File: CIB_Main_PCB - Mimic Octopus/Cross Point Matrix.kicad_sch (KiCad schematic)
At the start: 6 parts, among them J10 Ch 5-8, J11 Ch 9-12, J12 Ch 13-16, J13 Ch 17-20, J14 Ch 21-24, J9 Ch 1-4

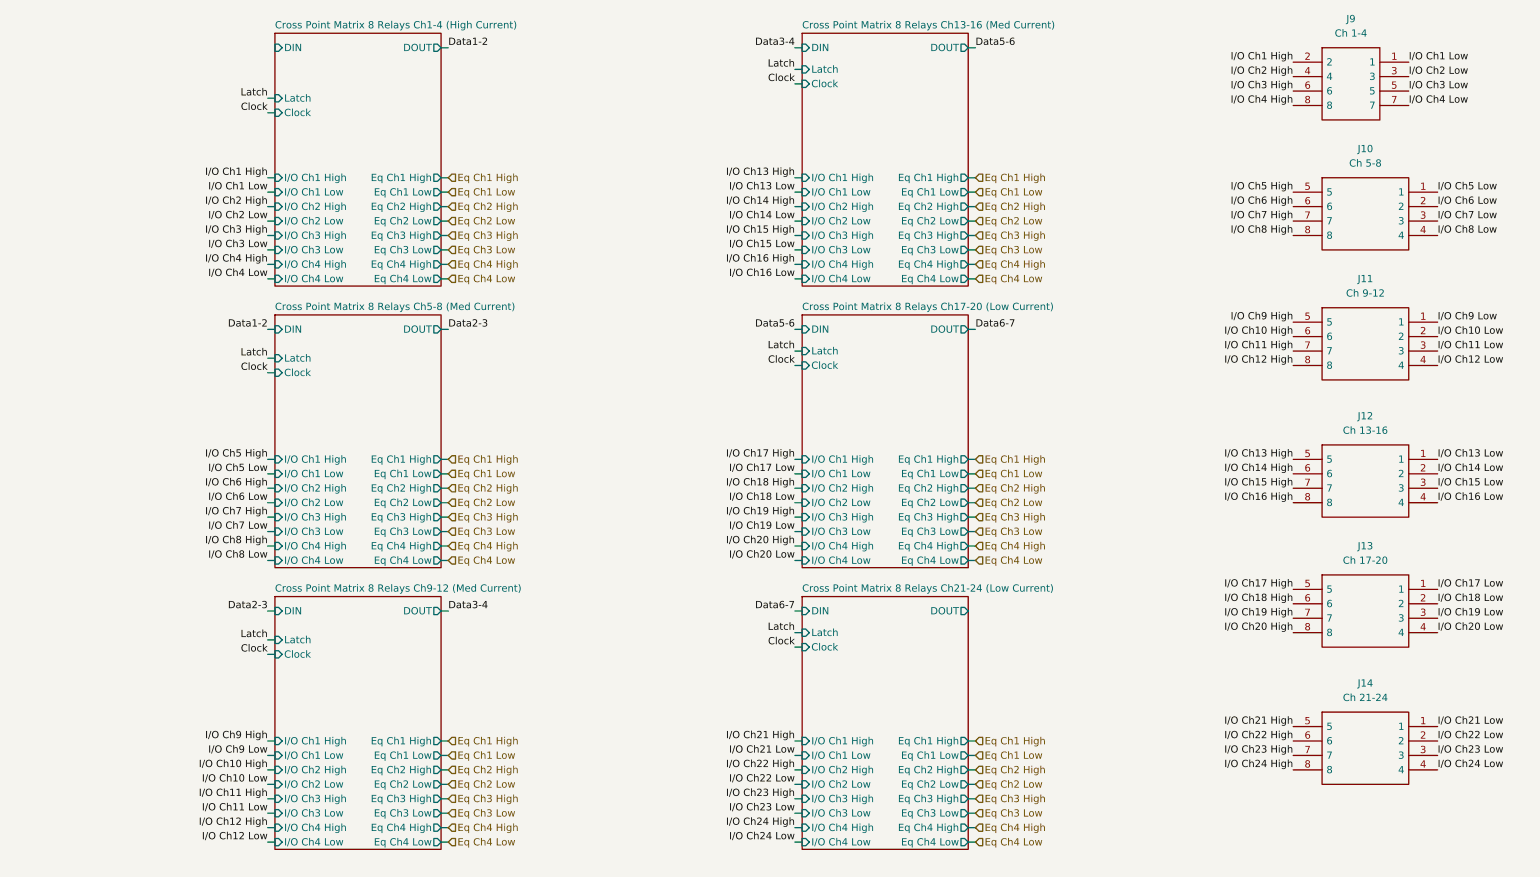
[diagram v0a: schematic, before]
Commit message: V0.1 PCB to be sent out
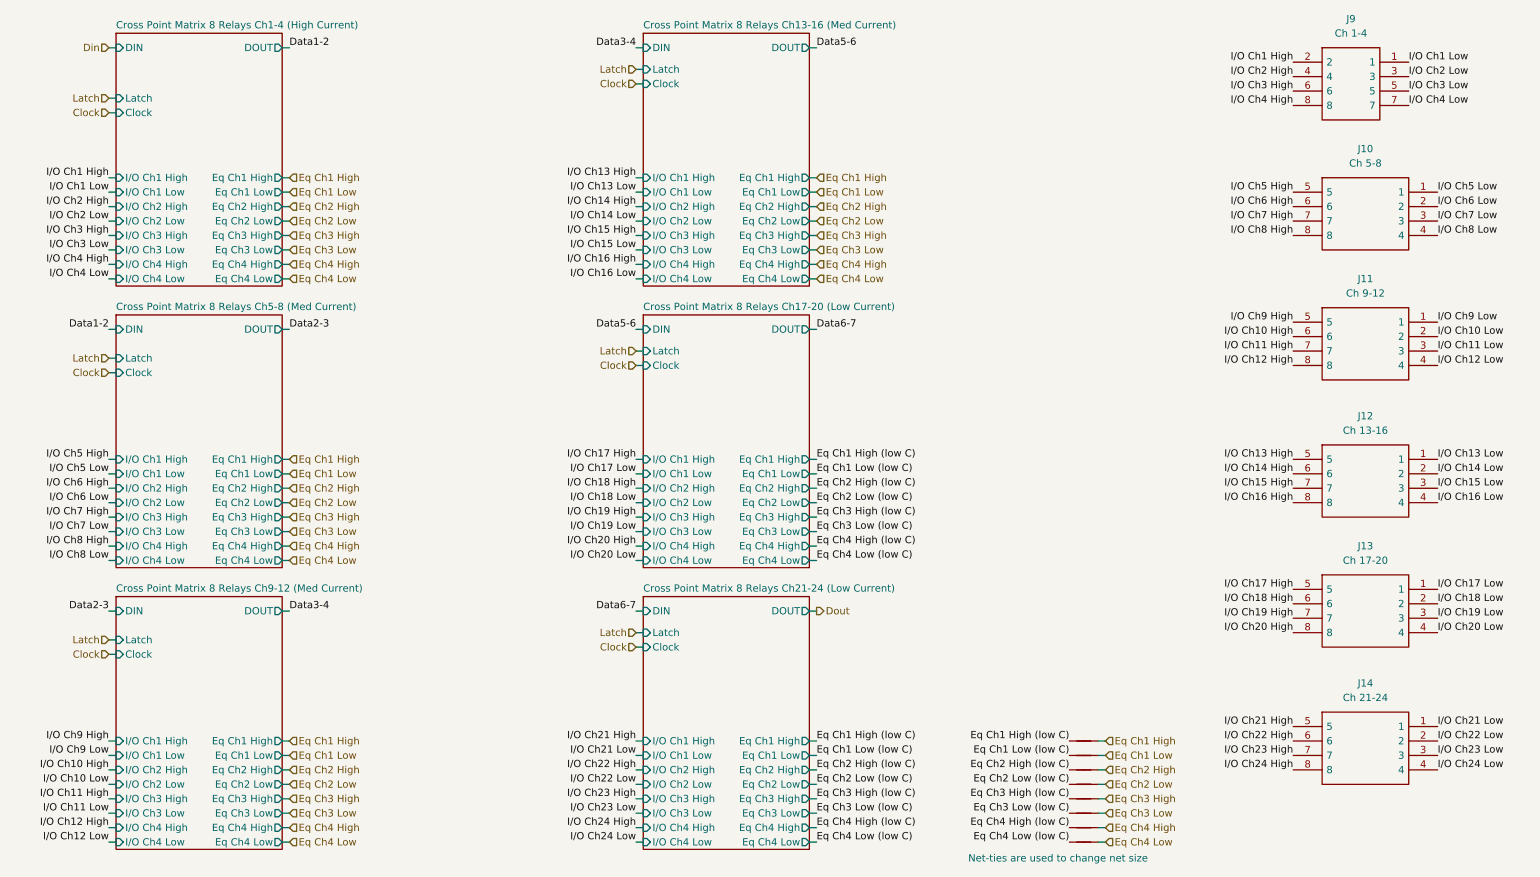
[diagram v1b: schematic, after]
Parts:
- added NT1, NT2, NT3, NT4, NT5, NT6, NT7, NT8: NetTie_2, NetTie:NetTie-2_SMD_Pad0.5mm, symbol Device:NetTie_2
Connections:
- net Eq Ch1 High: now also NT1.2
- net Eq Ch1 Low: now also NT2.2
- net Eq Ch2 High: now also NT3.2
- net Eq Ch2 Low: now also NT4.2
- net Eq Ch3 High: now also NT5.2
- net Eq Ch3 Low: now also NT6.2
- net Eq Ch4 High: now also NT7.2
- net Eq Ch4 Low: now also NT8.2
- new net Eq Ch1 High (low C): NT1.1
- new net Eq Ch1 Low (low C): NT2.1
- new net Eq Ch2 High (low C): NT3.1
- new net Eq Ch2 Low (low C): NT4.1
- new net Eq Ch3 High (low C): NT5.1
- new net Eq Ch3 Low (low C): NT6.1
- new net Eq Ch4 High (low C): NT7.1
- new net Eq Ch4 Low (low C): NT8.1
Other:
- note added: "Net-ties are used to change net size"

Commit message: BoM
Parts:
- J10, J11, J12, J13, J14: Manufacturer_Name Phoenix Contact -> (none); Manufacturer_Part_Number 1848668 -> (none); Mouser # (none) -> 651-1848668; Mouser Part Number 651-1848668 -> (none)
- J9: Manufacturer_Name Phoenix Contact -> (none); Manufacturer_Part_Number 1864095 -> (none); Mouser # (none) -> 651-1864095; Mouser Part Number 651-1864095 -> (none)
- NT1, NT2, NT3, NT4, NT5, NT6, NT7, NT8: dnp (none) -> dnp
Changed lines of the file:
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@@
+      (effects (font (size 1.27 1.27)) hide)
+    )
+    (property "dnp" "dnp" (id 4) (at 204.47 156.21 0)
       (effects (font (size 1.27 1.27)) hide)
     )
@@
       (effects (font (size 1.27 1.27)) (justify left) hide)
     )
-    (property "Manufacturer_Name" "Phoenix Contact" (id 6) (at 262.89 101.6 0)
-      (effects (font (size 1.27 1.27)) (justify left) hide)
-    )
-    (property "Manufacturer_Part_Number" "1848668" (id 7) (at 262.89 104.14 0)
-      (effects (font (size 1.27 1.27)) (justify left) hide)
-    )
-    (property "Mouser Part Number" "651-1848668" (id 8) (at 262.89 106.68 0)
+    (property "Manufacturer_Name" "" (id 6) (at 262.89 101.6 0)
+      (effects (font (size 1.27 1.27)) (justify left) hide)
+    )
+    (property "Manufacturer_Part_Number" "" (id 7) (at 262.89 104.14 0)
+      (effects (font (size 1.27 1.27)) (justify left) hide)
+    )
+    (property "Mouser Part Number" "" (id 8) (at 262.89 106.68 0)
       (effects (font (size 1.27 1.27)) (justify left) hide)
     )
@@
     )
     (property "Manufacturer #" "1848668" (id 13) (at 241.3 93.98 0)
+      (effects (font (size 1.27 1.27)) hide)
+    )
+    (property "Mouser #" "651-1848668" (id 14) (at 241.3 93.98 0)
       (effects (font (size 1.27 1.27)) hide)
     )
@@
       (effects (font (size 1.27 1.27)) (justify left) hide)
     )
-    (property "Manufacturer_Name" "Phoenix Contact" (id 6) (at 262.89 54.61 0)
-      (effects (font (size 1.27 1.27)) (justify left) hide)
-    )
-    (property "Manufacturer_Part_Number" "1848668" (id 7) (at 262.89 57.15 0)
-      (effects (font (size 1.27 1.27)) (justify left) hide)
-    )
-    (property "Mouser Part Number" "651-1848668" (id 8) (at 262.89 59.69 0)
+    (property "Manufacturer_Name" "" (id 6) (at 262.89 54.61 0)
+      (effects (font (size 1.27 1.27)) (justify left) hide)
+    )
+    (property "Manufacturer_Part_Number" "" (id 7) (at 262.89 57.15 0)
+      (effects (font (size 1.27 1.27)) (justify left) hide)
+    )
+    (property "Mouser Part Number" "" (id 8) (at 262.89 59.69 0)
       (effects (font (size 1.27 1.27)) (justify left) hide)
     )
@@
     )
     (property "Manufacturer #" "1848668" (id 13) (at 241.3 46.99 0)
+      (effects (font (size 1.27 1.27)) hide)
+    )
+    (property "Mouser #" "651-1848668" (id 14) (at 241.3 46.99 0)
       (effects (font (size 1.27 1.27)) hide)
     )
@@
       (effects (font (size 1.27 1.27)) hide)
     )
+    (property "dnp" "dnp" (id 4) (at 204.47 158.75 0)
+      (effects (font (size 1.27 1.27)) hide)
+    )
     (pin "1")
     (pin "2")
@@
       (effects (font (size 1.27 1.27)) hide)
     )
+    (property "dnp" "dnp" (id 4) (at 204.47 143.51 0)
+      (effects (font (size 1.27 1.27)) hide)
+    )
     (pin "1")
     (pin "2")
@@
       (effects (font (size 1.27 1.27)) hide)
     )
+    (property "dnp" "dnp" (id 4) (at 204.47 151.13 0)
+      (effects (font (size 1.27 1.27)) hide)
+    )
     (pin "1")
     (pin "2")
@@
       (effects (font (size 1.27 1.27)) hide)
     )
+    (property "dnp" "dnp" (id 4) (at 204.47 161.29 0)
+      (effects (font (size 1.27 1.27)) hide)
+    )
     (pin "1")
     (pin "2")
@@
     )
     (property "Datasheet" "~" (id 3) (at 204.47 153.67 0)
+      (effects (font (size 1.27 1.27)) hide)
+    )
+    (property "dnp" "dnp" (id 4) (at 204.47 153.67 0)
       (effects (font (size 1.27 1.27)) hide)
     )
@@
       (effects (font (size 1.27 1.27)) (justify left) hide)
     )
-    (property "Manufacturer_Name" "Phoenix Contact" (id 6) (at 262.89 124.46 0)
-      (effects (font (size 1.27 1.27)) (justify left) hide)
-    )
-    (property "Manufacturer_Part_Number" "1848668" (id 7) (at 262.89 127 0)
-      (effects (font (size 1.27 1.27)) (justify left) hide)
-    )
-    (property "Mouser Part Number" "651-1848668" (id 8) (at 262.89 129.54 0)
+    (property "Manufacturer_Name" "" (id 6) (at 262.89 124.46 0)
+      (effects (font (size 1.27 1.27)) (justify left) hide)
+    )
+    (property "Manufacturer_Part_Number" "" (id 7) (at 262.89 127 0)
+      (effects (font (size 1.27 1.27)) (justify left) hide)
+    )
+    (property "Mouser Part Number" "" (id 8) (at 262.89 129.54 0)
       (effects (font (size 1.27 1.27)) (justify left) hide)
     )
@@
     )
     (property "Manufacturer #" "1848668" (id 13) (at 241.3 116.84 0)
+      (effects (font (size 1.27 1.27)) hide)
+    )
+    (property "Mouser #" "651-1848668" (id 14) (at 241.3 116.84 0)
       (effects (font (size 1.27 1.27)) hide)
     )
@@
       (effects (font (size 1.27 1.27)) (justify left) hide)
     )
-    (property "Description" "Push spring connector 5mm pitch 8 way Phoenix Contact SDC Series 5mm Pitch Straight Pluggable Terminal Block, Plug with Plug In Termination, PCB Mount, 8 Way" (id 4) (at 257.81 26.67 0)
+    (property "Description" "Pluggable Terminal Blocks SDDC 1,5/ 4-PV-3,5" (id 4) (at 257.81 26.67 0)
       (effects (font (size 1.27 1.27)) (justify left) hide)
     )
@@
       (effects (font (size 1.27 1.27)) (justify left) hide)
     )
-    (property "Manufacturer_Name" "Phoenix Contact" (id 6) (at 257.81 31.75 0)
-      (effects (font (size 1.27 1.27)) (justify left) hide)
-    )
-    (property "Manufacturer_Part_Number" "1864095" (id 7) (at 257.81 34.29 0)
-      (effects (font (size 1.27 1.27)) (justify left) hide)
-    )
-    (property "Mouser Part Number" "651-1864095" (id 8) (at 257.81 36.83 0)
+    (property "Manufacturer_Name" "" (id 6) (at 257.81 31.75 0)
+      (effects (font (size 1.27 1.27)) (justify left) hide)
+    )
+    (property "Manufacturer_Part_Number" "" (id 7) (at 257.81 34.29 0)
+      (effects (font (size 1.27 1.27)) (justify left) hide)
+    )
+    (property "Mouser Part Number" "" (id 8) (at 257.81 36.83 0)
       (effects (font (size 1.27 1.27)) (justify left) hide)
     )
@@
     )
     (property "Manufacturer #" "1864095" (id 13) (at 241.3 24.13 0)
+      (effects (font (size 1.27 1.27)) hide)
+    )
+    (property "Mouser #" "651-1864095" (id 14) (at 241.3 24.13 0)
       (effects (font (size 1.27 1.27)) hide)
     )
@@
       (effects (font (size 1.27 1.27)) hide)
     )
+    (property "dnp" "dnp" (id 4) (at 204.47 146.05 0)
+      (effects (font (size 1.27 1.27)) hide)
+    )
     (pin "1")
     (pin "2")
@@
       (effects (font (size 1.27 1.27)) (justify left) hide)
     )
-    (property "Manufacturer_Name" "Phoenix Contact" (id 6) (at 262.89 148.59 0)
-      (effects (font (size 1.27 1.27)) (justify left) hide)
-    )
-    (property "Manufacturer_Part_Number" "1848668" (id 7) (at 262.89 151.13 0)
-      (effects (font (size 1.27 1.27)) (justify left) hide)
-    )
-    (property "Mouser Part Number" "651-1848668" (id 8) (at 262.89 153.67 0)
+    (property "Manufacturer_Name" "" (id 6) (at 262.89 148.59 0)
+      (effects (font (size 1.27 1.27)) (justify left) hide)
+    )
+    (property "Manufacturer_Part_Number" "" (id 7) (at 262.89 151.13 0)
+      (effects (font (size 1.27 1.27)) (justify left) hide)
+    )
+    (property "Mouser Part Number" "" (id 8) (at 262.89 153.67 0)
       (effects (font (size 1.27 1.27)) (justify left) hide)
     )
@@
     )
     (property "Manufacturer #" "1848668" (id 13) (at 241.3 140.97 0)
+      (effects (font (size 1.27 1.27)) hide)
+    )
+    (property "Mouser #" "651-1848668" (id 14) (at 241.3 140.97 0)
       (effects (font (size 1.27 1.27)) hide)
     )
@@
       (effects (font (size 1.27 1.27)) hide)
     )
+    (property "dnp" "dnp" (id 4) (at 204.47 148.59 0)
+      (effects (font (size 1.27 1.27)) hide)
+    )
     (pin "1")
     (pin "2")
@@
       (effects (font (size 1.27 1.27)) (justify left) hide)
     )
-    (property "Manufacturer_Name" "Phoenix Contact" (id 6) (at 262.89 77.47 0)
-      (effects (font (size 1.27 1.27)) (justify left) hide)
-    )
-    (property "Manufacturer_Part_Number" "1848668" (id 7) (at 262.89 80.01 0)
-      (effects (font (size 1.27 1.27)) (justify left) hide)
-    )
-    (property "Mouser Part Number" "651-1848668" (id 8) (at 262.89 82.55 0)
+    (property "Manufacturer_Name" "" (id 6) (at 262.89 77.47 0)
+      (effects (font (size 1.27 1.27)) (justify left) hide)
+    )
+    (property "Manufacturer_Part_Number" "" (id 7) (at 262.89 80.01 0)
+      (effects (font (size 1.27 1.27)) (justify left) hide)
+    )
+    (property "Mouser Part Number" "" (id 8) (at 262.89 82.55 0)
       (effects (font (size 1.27 1.27)) (justify left) hide)
     )
@@
       (effects (font (size 1.27 1.27)) hide)
     )
+    (property "Mouser #" "651-1848668" (id 14) (at 241.3 69.85 0)
+      (effects (font (size 1.27 1.27)) hide)
+    )
